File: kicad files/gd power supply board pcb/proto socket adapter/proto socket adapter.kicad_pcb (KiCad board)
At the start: 2 copper layers, 39.9 x 27.4 mm, 4 parts, among them J1 Right Angle, J2 Rev2 Header, J3 RP2040 Header, J4 Straight

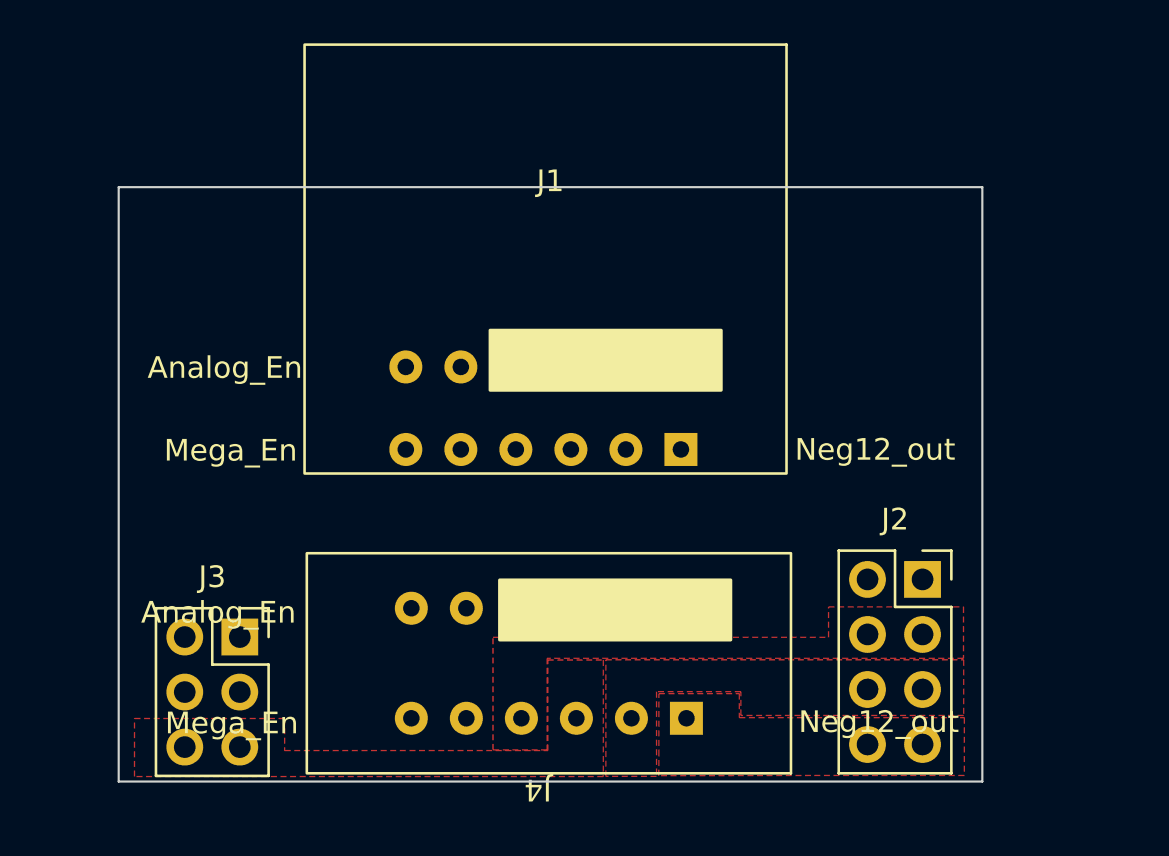
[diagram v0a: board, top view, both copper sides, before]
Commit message: sub rev1 to fab
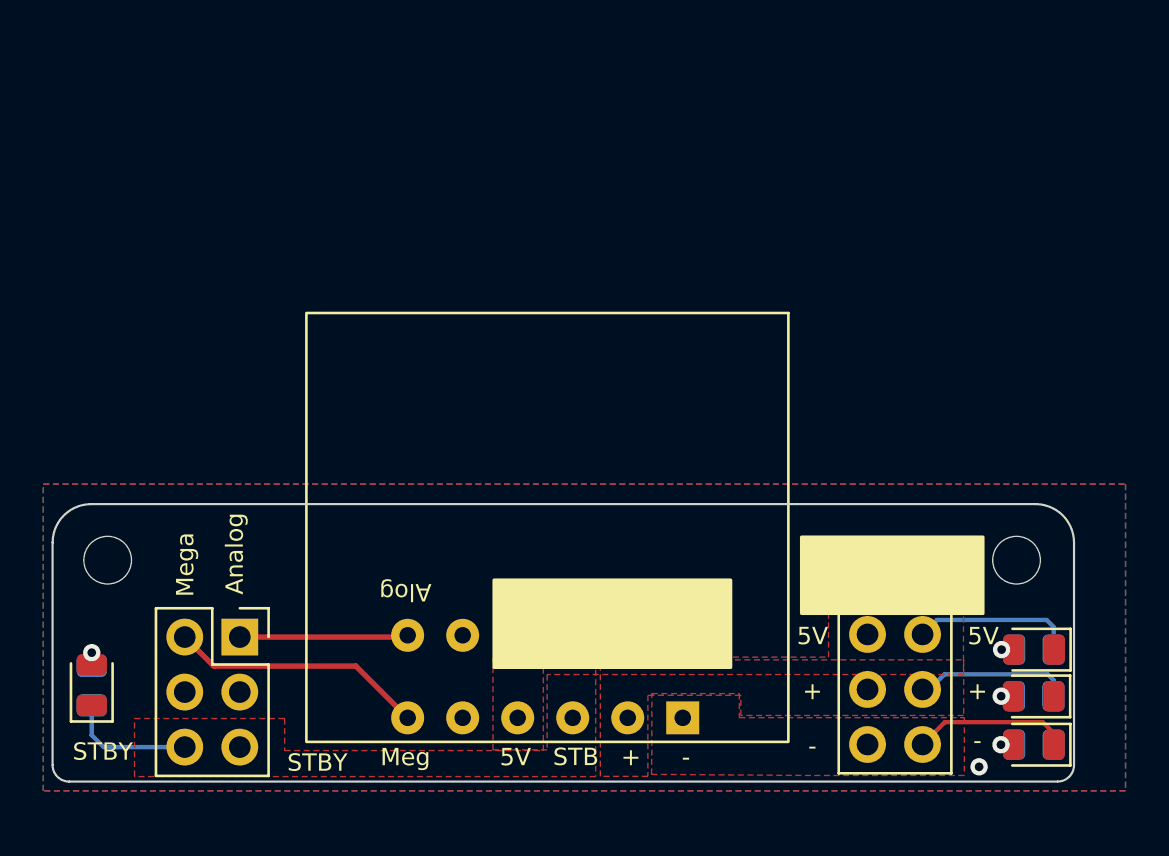
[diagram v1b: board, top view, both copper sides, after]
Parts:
- removed J4: Straight, My Libraries:Sullins-EBC06DCWN-Edge Socket 12 pos (6x2)
- added D1: -12v, LED_SMD:LED_0805_2012Metric, F.Cu at (169.0, 127.4)
- added D2: +12v, LED_SMD:LED_0805_2012Metric, F.Cu at (169.0, 125.2)
- added D3: Mega, LED_SMD:LED_0805_2012Metric, F.Cu at (169.0, 123.0)
- added D4: Stby, LED_SMD:LED_0805_2012Metric, F.Cu at (125.5, 124.7)
- added H1: MountingHole, MountingHole:MountingHole_2.2mm_M2, F.Cu at (126.2, 118.9)
- added H2: MountingHole, MountingHole:MountingHole_2.2mm_M2, F.Cu at (168.2, 118.9)
- added R1: 1K, Resistor_SMD:R_0805_2012Metric, B.Cu at (169.0, 127.4)
- added R2: 1K, Resistor_SMD:R_0805_2012Metric, B.Cu at (169.0, 125.2)
- added R3: 1K, Resistor_SMD:R_0805_2012Metric, B.Cu at (125.5, 124.7)
- added R4: 1K, Resistor_SMD:R_0805_2012Metric, B.Cu at (169.0, 123.0)
- moved J1 12.4 mm to (146.5, 117.2)
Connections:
- J1 pad 2: /GND -> GND
- J1 pad 4: /GND -> GND
- J1 pad 6: /GND -> GND
- J1 pad 8: /GND -> GND
- J2 pad 1: /GND -> GND
- J2 pad 2: /GND -> GND
- J3 pad 1: /GND -> /Analog_En
- J3 pad 2: /GND -> /Mega_En
- J3 pad 3: /stb_5v -> GND
- J3 pad 4: /stb_5v -> GND
- J3 pad 5: /Mega_En -> /stb_5v
- J3 pad 6: /Analog_En -> /stb_5v
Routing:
- net /Mega_En: track 0.00 -> 11.8 mm
- net /Analog_En: track 0.00 -> 7.67 mm
- net /mega_5v: track 0.00 -> 7.51 mm
- net /Pos12_Out: track 0.00 -> 6.87 mm
- net /Neg12_Out: track 0.00 -> 6.72 mm
- net /stb_5v: track 0.00 -> 5.90 mm
- net Net-(D1-Pad2): track 0.00 -> 1.19 mm, vias 0 -> 1
- net Net-(D4-Pad2): track 0.00 -> 1.17 mm, vias 0 -> 1
- net Net-(D3-Pad2): track 0.00 -> 1.14 mm, vias 0 -> 1
- net Net-(D2-Pad2): track 0.00 -> 1.14 mm, vias 0 -> 1
- net GND: vias 0 -> 1
- added copper zone on B.Cu, net GND
- added copper zone on F.Cu, net GND
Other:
- board size 39.9 x 27.4 mm -> 47.2 x 12.8 mm
- board text added: "+"
- board text added: "-"
- board text added: "5V"
- board text added: "Alog"
- board text added: "Analog"
- board text added: "Meg"
- board text added: "Mega"
- board text added: "STB"
- board text added: "STBY"
- board text added: "gd-proto adapter rev1 2022-04-07"
- board text removed: "Analog_En"
- board text removed: "Mega_En"
- board text removed: "Neg12_out"
